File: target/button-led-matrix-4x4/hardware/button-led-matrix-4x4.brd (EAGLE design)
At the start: 23 parts, among them IC1 ATMEGA48/88/168-AU, X1 CRYSTALS-NOGND-HC49

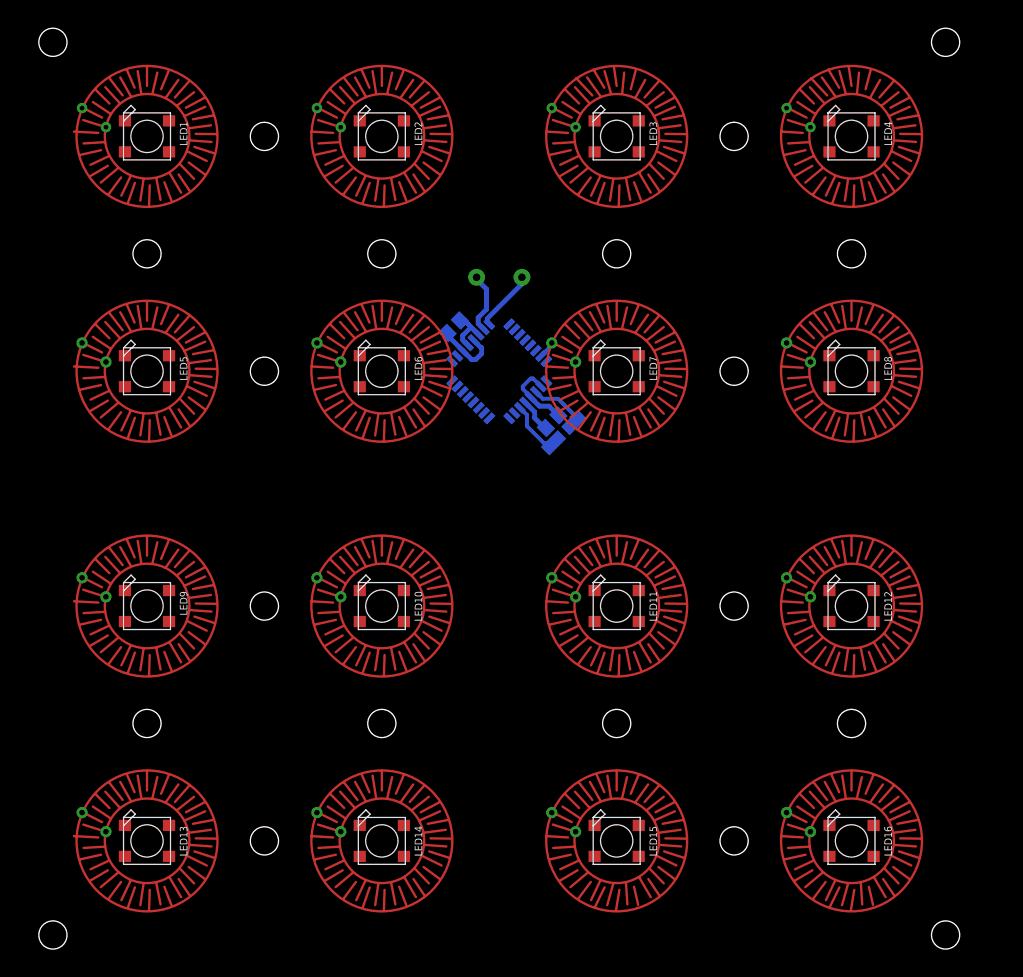
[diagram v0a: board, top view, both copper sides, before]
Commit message: button-led-matrix-4x4 hardware
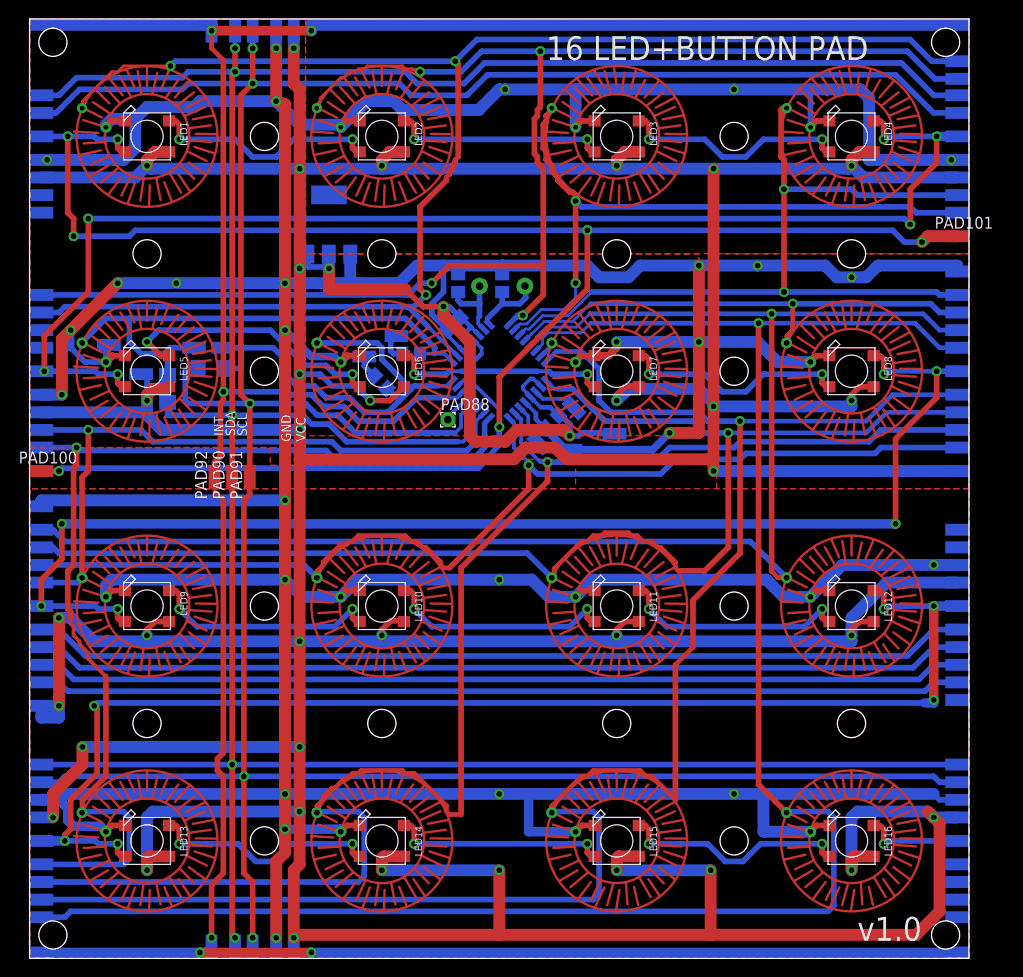
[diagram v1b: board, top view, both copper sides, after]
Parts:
- added C3, C4: 18, rcl:C0805
- added IC2: AMS1117-3.3, burr-brown:SOT223
- added PAD10, PAD100, PAD101, PAD102, PAD103, PAD104, PAD105, PAD11, PAD12, PAD13, PAD14, PAD15, PAD16, PAD17, PAD18, PAD19, PAD20, PAD21, PAD22, PAD23, PAD24, PAD25, PAD26, PAD27, PAD28, PAD29, PAD3, PAD30, PAD31, PAD32, PAD33, PAD34, PAD35, PAD36, PAD37, PAD38, PAD39, PAD4, PAD40, PAD41, PAD42, PAD43, PAD44, PAD45, PAD46, PAD47, PAD48, PAD49, PAD5, PAD50, PAD51, PAD52, PAD53, PAD54, PAD55, PAD56, PAD57, PAD58, PAD59, PAD6, PAD60, PAD61, PAD62, PAD63, PAD64, PAD65, PAD66, PAD67, PAD68, PAD69, PAD7, PAD70, PAD71, PAD72, PAD73, PAD74, PAD75, PAD76, PAD77, PAD78, PAD79, PAD8, PAD80, PAD81, PAD82, PAD83, PAD84, PAD85, PAD86, PAD87, PAD89, PAD9, PAD90, PAD91, PAD92, PAD93, PAD94, PAD95, PAD96, PAD97, PAD98, PAD99: WIREPADSMD1,27-254, wirepad:SMD1,27-2,54
- added PAD88: (no value), wirepad:1,6/0,8
- added R1, R2: (no value), rcl:R1206
- added R3, R4: (no value), rcl:R0805
- moved PAD2 1.59 mm to (54.2, 54.8), turned to 315 degrees
- moved PAD1 1.54 mm to (58.0, 58.6), turned to 135 degrees
- moved X1 0.99 mm to (50.3, 71.6)
- moved C2 0.31 mm to (45.2, 67.6)
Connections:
- removed net N$11: IC1.9
- removed net N$13: IC1.11
- removed net N$14: IC1.12
- removed net N$15: IC1.13
- removed net N$16: IC1.14
- removed net N$18: IC1.16
- removed net N$19: IC1.17
- removed net N$32: S1.SIG7
- removed net N$65: LED5.3-GND
- removed net N$66: LED6.3-GND
- removed net N$67: LED7.3-GND
- removed net N$68: LED8.3-GND
- removed net N$7: IC1.30
- removed net N$9: IC1.1
- new net INT: IC1.30, PAD67.1, PAD68.1, PAD69.1, PAD70.1, PAD71.1, PAD72.1, PAD92.1
- new net N$17: PAD98.1, R4.2
- new net N$20: PAD79.1
- new net XTAL1: C4.2, IC1.7, X1.2
- new net XTAL2: C3.2, IC1.8, X1.1
- net B1: now also IC1.2, PAD18.1, PAD89.1
- net B10: now also IC1.24, PAD23.1, PAD32.1
- net B11: now also IC1.17, PAD25.1, PAD33.1
- net B12: now also IC1.13, PAD28.1, PAD34.1
- net B13: now also IC1.25, PAD12.1, PAD38.1
- net B14: now also IC1.23, PAD24.1, PAD37.1
- net B15: now also IC1.16, PAD26.1, PAD36.1
- net B16: now also IC1.14, PAD27.1, PAD35.1
- net B2: now also IC1.9, PAD13.1, PAD17.1
- net B3: now also IC1.10, PAD15.1
- net B4: now also IC1.11, PAD16.1, PAD30.1
- net B5: now also IC1.1, PAD103.1, R2.2, R4.1
- net B6: now also IC1.32, PAD102.1, R1.2, R3.1
- net B8: now also IC1.12, PAD29.1
- net B9: now also IC1.26, PAD11.1, PAD31.1
- net DATA: now also PAD100.1, PAD101.1, PAD7.1
- net DO12: now also PAD10.1, PAD5.1
- net DO4: now also PAD3.1, PAD8.1
- net DO8: now also PAD4.1, PAD9.1
- net D_OUT: now also PAD6.1
- net GND: now also C3.1, C4.1, IC2.1, LED5.3-GND, LED6.3-GND, LED7.3-GND, LED8.3-GND, PAD105.1, PAD44.1, PAD45.1, PAD50.1, PAD53.1, PAD58.1, PAD61.1, PAD65.1, PAD75.1, PAD87.1, PAD93.1, PAD95.1, S1.SIG7
- net N$1: now also PAD86.1; no longer IC1.7, X1.2
- net N$10: now also PAD99.1; no longer IC1.2
- net N$12: now also PAD47.1; no longer IC1.10
- net N$2: now also PAD97.1, R3.2; no longer IC1.8, X1.1
- net N$3: now also PAD19.1, PAD39.1; no longer IC1.23
- net N$4: now also PAD20.1, PAD40.1; no longer IC1.24
- net N$5: now also PAD21.1, PAD41.1; no longer IC1.25
- net N$6: now also PAD22.1, PAD42.1; no longer IC1.26
- net N$8: now also PAD43.1; no longer IC1.32
- net RESET: now also PAD88.1
- net SCL: now also PAD51.1, PAD56.1, PAD60.1, PAD64.1, PAD73.1, PAD82.1, PAD91.1, R1.1
- net SDA: now also PAD52.1, PAD55.1, PAD59.1, PAD63.1, PAD74.1, PAD81.1, PAD90.1, R2.1
- net VCC: now also IC2.2, IC2.3, PAD104.1, PAD46.1, PAD48.1, PAD49.1, PAD54.1, PAD57.1, PAD62.1, PAD66.1, PAD76.1, PAD83.1, PAD94.1, PAD96.1
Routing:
- net VCC: track 13.1 -> 804.2 mm, vias 0 -> 38
- net GND: track 10.8 -> 724.1 mm, vias 0 -> 26
- net SCL: track 0.00 -> 338.5 mm, vias 0 -> 5
- net SDA: track 0.00 -> 335.0 mm, vias 0 -> 5
- net INT: track 0.00 -> 325.6 mm, vias 0 -> 6
- net DATA: track 0.00 -> 200.7 mm, vias 0 -> 7
- net B16: track 0.00 -> 200.5 mm, vias 0 -> 1
- net B15: track 0.00 -> 183.4 mm, vias 0 -> 1
- net B1: track 0.00 -> 173.6 mm, vias 0 -> 3
- net B14: track 0.00 -> 160.0 mm, vias 0 -> 1
- net B2: track 0.00 -> 159.2 mm, vias 0 -> 4
- net B12: track 0.00 -> 158.4 mm, vias 0 -> 1
- net DO12: track 0.00 -> 140.4 mm, vias 0 -> 6
- net B11: track 0.00 -> 139.8 mm, vias 0 -> 1
- net DO8: track 0.00 -> 139.5 mm, vias 0 -> 6
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- added copper zone on layer 1, net GND
- added copper zone on layer 16, net VCC
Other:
- board outline added: 100 x 100 mm
- board text added: "16 LED+BUTTON PAD"
- board text added: "ADC6"
- board text added: "ADC7"
- board text added: "AMS1117-3.3"
- board text added: "B1"
- board text added: "B10"
- board text added: "B11"
- board text added: "B12"
- board text added: "B13"
- board text added: "B14"
- board text added: "B15"
- board text added: "B16"
- board text added: "B2"
- board text added: "B3"
- board text added: "B4"
- board text added: "B9"
- board text added: "CUT"
- board text added: "DATA"
- board text added: "DOUT"
- board text added: "GND"
- board text added: "I"
- board text added: "INT"
- board text added: "MISO"
- board text added: "MOSI"
- board text added: "ONLY FOR USB DEVICE"
- board text added: "RESET"
- board text added: "SCK"
- board text added: "SCL"
- board text added: "SDA"
- board text added: "VCC"
- board text added: "v1.0"
